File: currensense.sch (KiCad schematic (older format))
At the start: 8 parts, among them U801 LM358

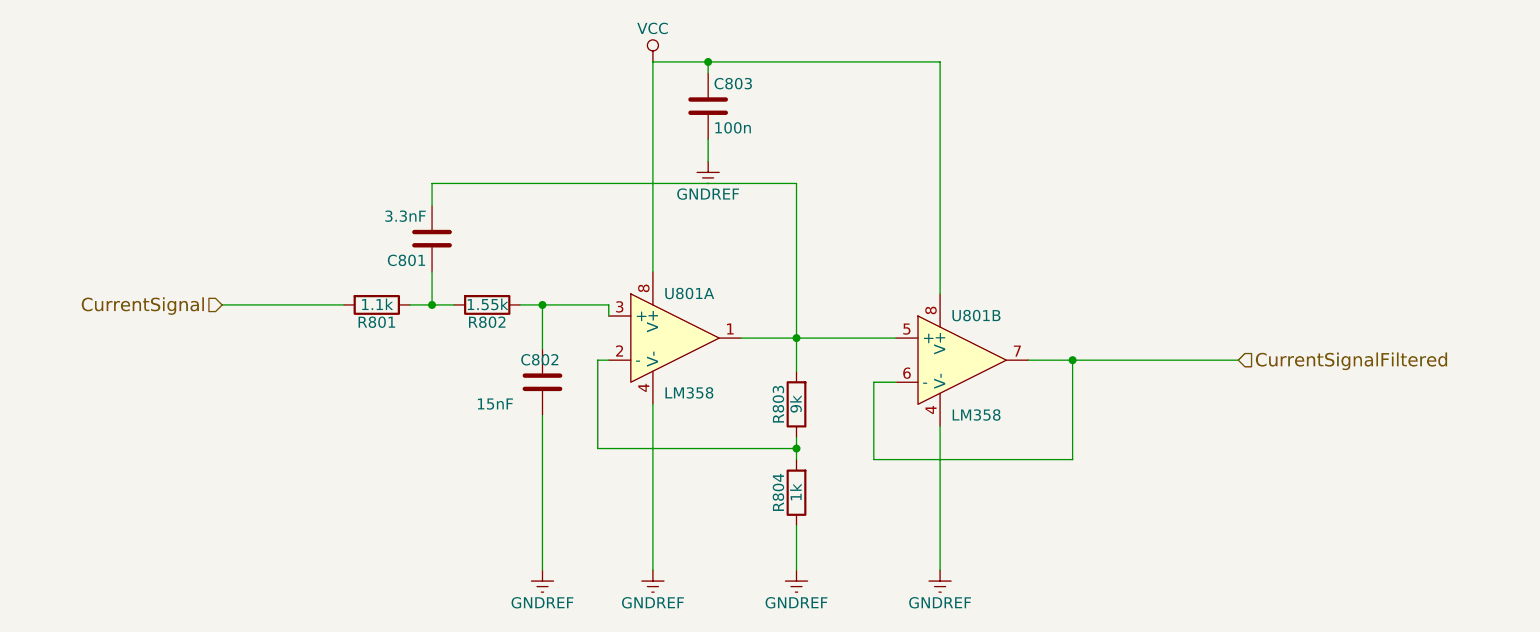
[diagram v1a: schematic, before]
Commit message: New amplifiers, fuse and general mayhem
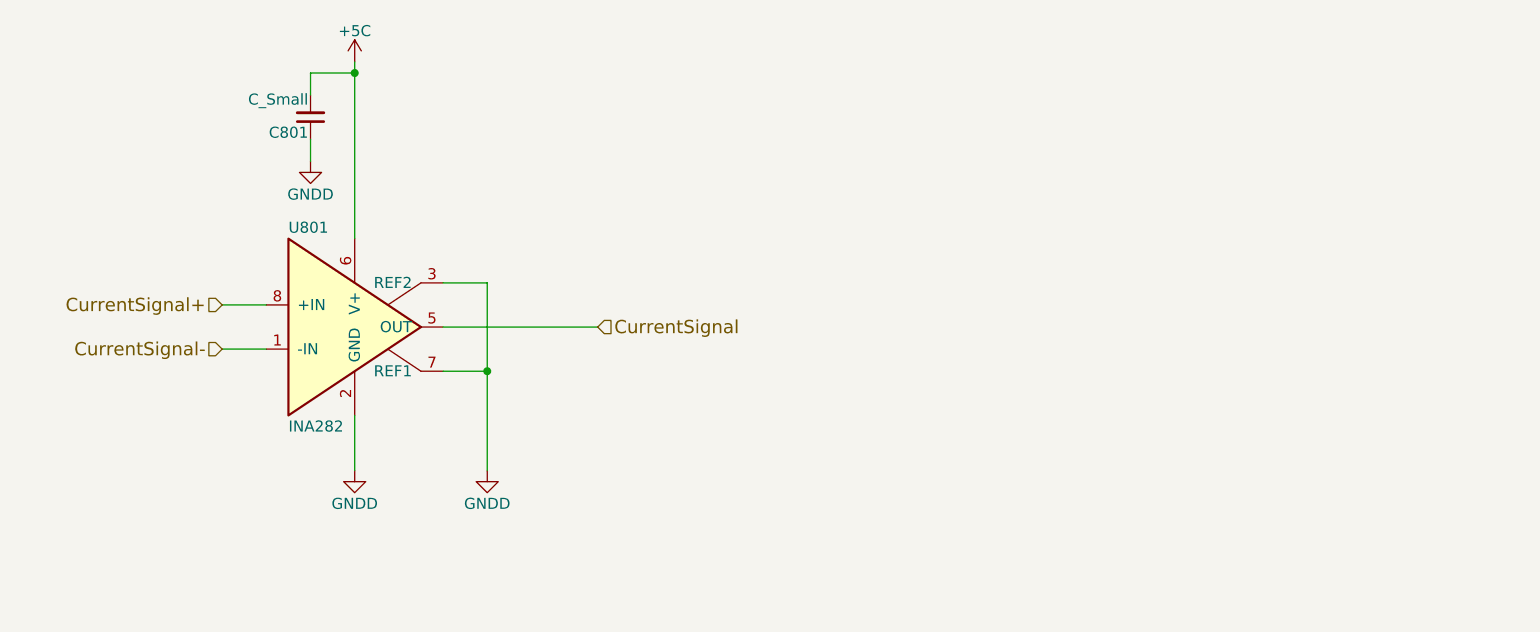
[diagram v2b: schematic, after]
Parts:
- removed C801: 3.3nF, Capacitors_SMD:C_0805, symbol C
- removed C802: 15nF, Capacitors_SMD:C_0805, symbol C
- removed C803: 100n, Capacitors_SMD:C_0805, symbol C
- removed R801: 1.1k, Resistors_SMD:R_0603, symbol R
- removed R802: 1.55k, Resistors_SMD:R_0603, symbol R
- removed R803: 9k, Resistors_SMD:R_0603, symbol R
- removed R804: 1k, Resistors_SMD:R_0603, symbol R
- removed U801: LM358, Housings_SOIC:SOIC-8_3.9x4.9mm_Pitch1.27mm, symbol LM358
- added C801: C_Small, axel:C_0603_CustomText, symbol C_Small
- added U801: INA282, Housings_SOIC:SOIC-8_3.9x4.9mm_Pitch1.27mm, symbol INA282
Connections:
- net CurrentSignal: now also U801.5 (OUT)
- new net +5C: C801.2, U801.6 (V+)
- new net CurrentSignal+: U801.8 (+IN)
- new net CurrentSignal-: U801.1 (-IN)
- new net GNDD: C801.1, U801.2 (GND), U801.3 (REF2), U801.7 (REF1)
